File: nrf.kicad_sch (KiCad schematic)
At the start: 25 parts, among them J1 USB_C_Receptacle_USB2.0_16P, SW1 RESET, U1 nRF52840, U2 BQ25101YFPR, Y1 32.768kHz, Y2 32mHz

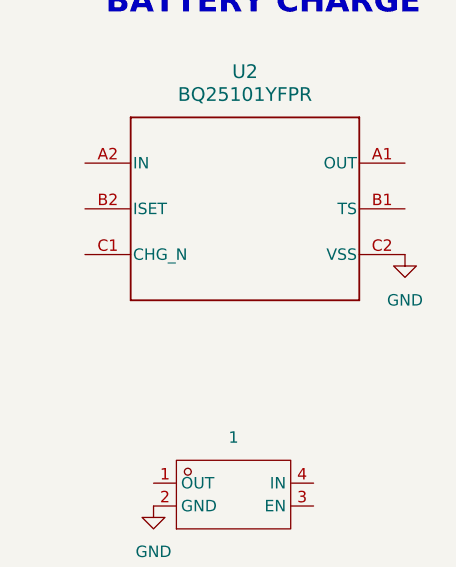
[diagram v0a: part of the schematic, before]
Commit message: test windows 3
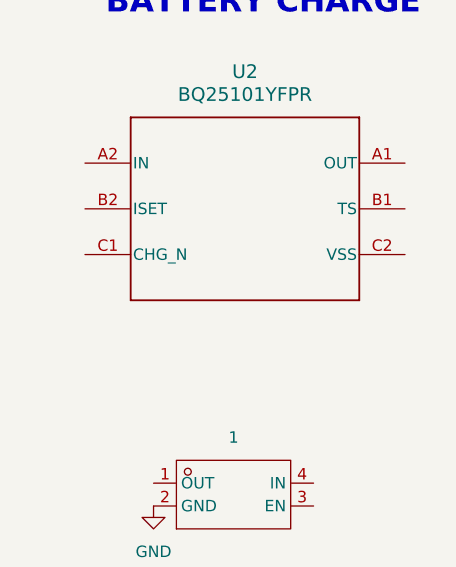
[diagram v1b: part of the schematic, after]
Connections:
- net GND: no longer U2.C2 (VSS)
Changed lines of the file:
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@@
-	(symbol
-		(lib_id "power:GND")
-		(at 236.22 59.69 0)
-		(unit 1)
-		(body_style 1)
-		(exclude_from_sim no)
-		(in_bom yes)
-		(on_board yes)
-		(in_pos_files yes)
-		(dnp no)
-		(fields_autoplaced yes)
-		(property "Reference" "#PWR022"
-			(at 236.22 66.04 0)
-			(hide yes)
-			(show_name no)
-			(do_not_autoplace no)
-			(effects
-				(font
-					(size 1.27 1.27)
-				)
-			)
-		)
-		(property "Value" "GND"
-			(at 236.22 64.77 0)
-			(show_name no)
-			(do_not_autoplace no)
-			(effects
-				(font
-					(size 1.27 1.27)
-				)
-			)
-		)
-		(property "Footprint" ""
-			(at 236.22 59.69 0)
-			(hide yes)
-			(show_name no)
-			(do_not_autoplace no)
-			(effects
-				(font
-					(size 1.27 1.27)
-				)
-			)
-		)
-		(property "Datasheet" ""
-			(at 236.22 59.69 0)
-			(hide yes)
-			(show_name no)
-			(do_not_autoplace no)
-			(effects
-				(font
-					(size 1.27 1.27)
-				)
-			)
-		)
-		(property "Description" "Power symbol creates a global label with name \"GND\" , ground"
-			(at 236.22 59.69 0)
-			(hide yes)
-			(show_name no)
-			(do_not_autoplace no)
-			(effects
-				(font
-					(size 1.27 1.27)
-				)
-			)
-		)
-		(pin "1"
-		)
-		(instances
-			(project "nrf"
-				(path "/0c64da4f-9d5f-4fc8-ac76-7e5704c1497b"
-					(reference "#PWR022")
-					(unit 1)
-				)
-			)
-		)
-	)
 	(symbol
 		(lib_id "power:GND")

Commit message: Test na windows 2
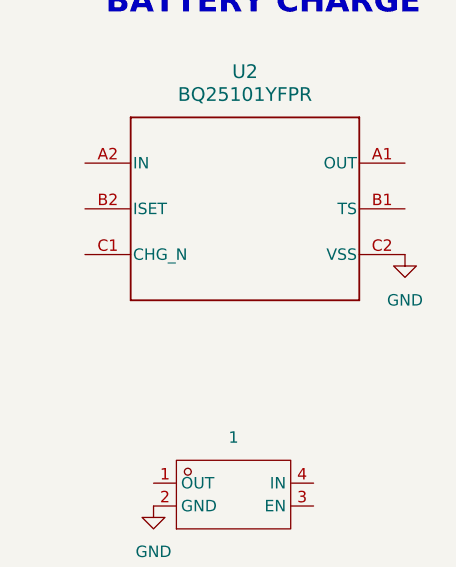
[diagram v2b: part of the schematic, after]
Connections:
- net GND: now also U2.C2 (VSS)
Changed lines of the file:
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@@
+	(symbol
+		(lib_id "power:GND")
+		(at 236.22 59.69 0)
+		(unit 1)
+		(body_style 1)
+		(exclude_from_sim no)
+		(in_bom yes)
+		(on_board yes)
+		(in_pos_files yes)
+		(dnp no)
+		(fields_autoplaced yes)
+		(property "Reference" "#PWR022"
+			(at 236.22 66.04 0)
+			(hide yes)
+			(show_name no)
+			(do_not_autoplace no)
+			(effects
+				(font
+					(size 1.27 1.27)
+				)
+			)
+		)
+		(property "Value" "GND"
+			(at 236.22 64.77 0)
+			(show_name no)
+			(do_not_autoplace no)
+			(effects
+				(font
+					(size 1.27 1.27)
+				)
+			)
+		)
+		(property "Footprint" ""
+			(at 236.22 59.69 0)
+			(hide yes)
+			(show_name no)
+			(do_not_autoplace no)
+			(effects
+				(font
+					(size 1.27 1.27)
+				)
+			)
+		)
+		(property "Datasheet" ""
+			(at 236.22 59.69 0)
+			(hide yes)
+			(show_name no)
+			(do_not_autoplace no)
+			(effects
+				(font
+					(size 1.27 1.27)
+				)
+			)
+		)
+		(property "Description" "Power symbol creates a global label with name \"GND\" , ground"
+			(at 236.22 59.69 0)
+			(hide yes)
+			(show_name no)
+			(do_not_autoplace no)
+			(effects
+				(font
+					(size 1.27 1.27)
+				)
+			)
+		)
+		(pin "1"
+		)
+		(instances
+			(project "nrf"
+				(path "/0c64da4f-9d5f-4fc8-ac76-7e5704c1497b"
+					(reference "#PWR022")
+					(unit 1)
+				)
+			)
+		)
+	)
 	(symbol
 		(lib_id "power:GND")
